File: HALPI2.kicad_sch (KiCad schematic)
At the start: 0 parts

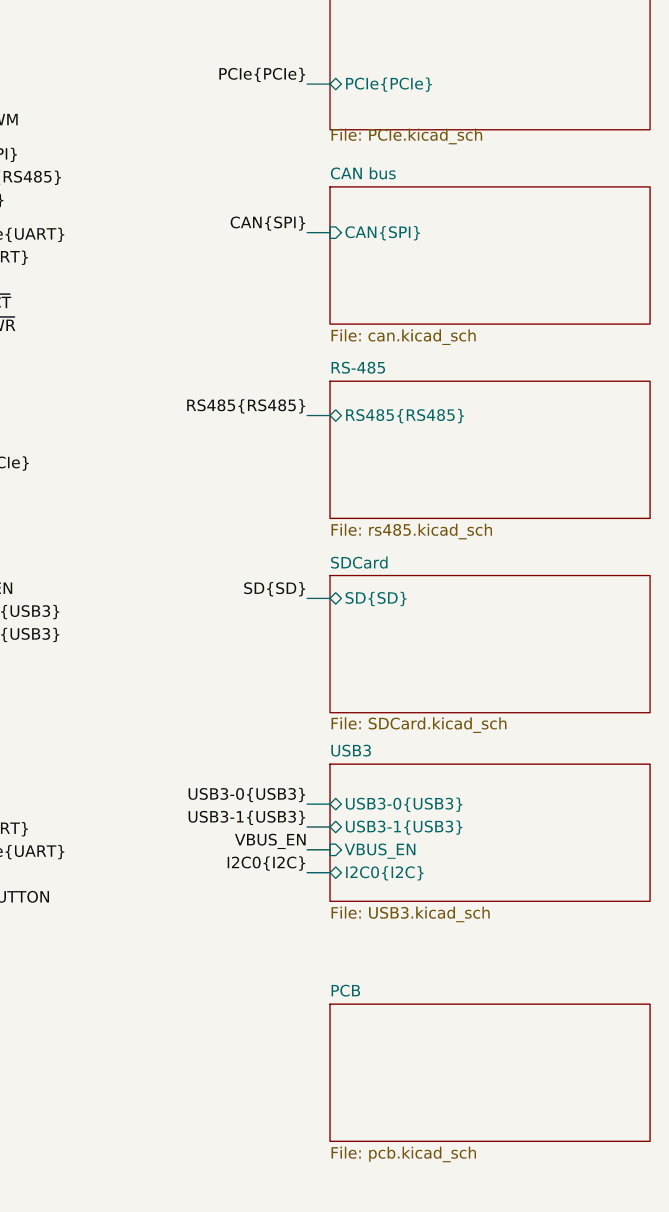
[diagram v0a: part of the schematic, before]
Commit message: Route more traces
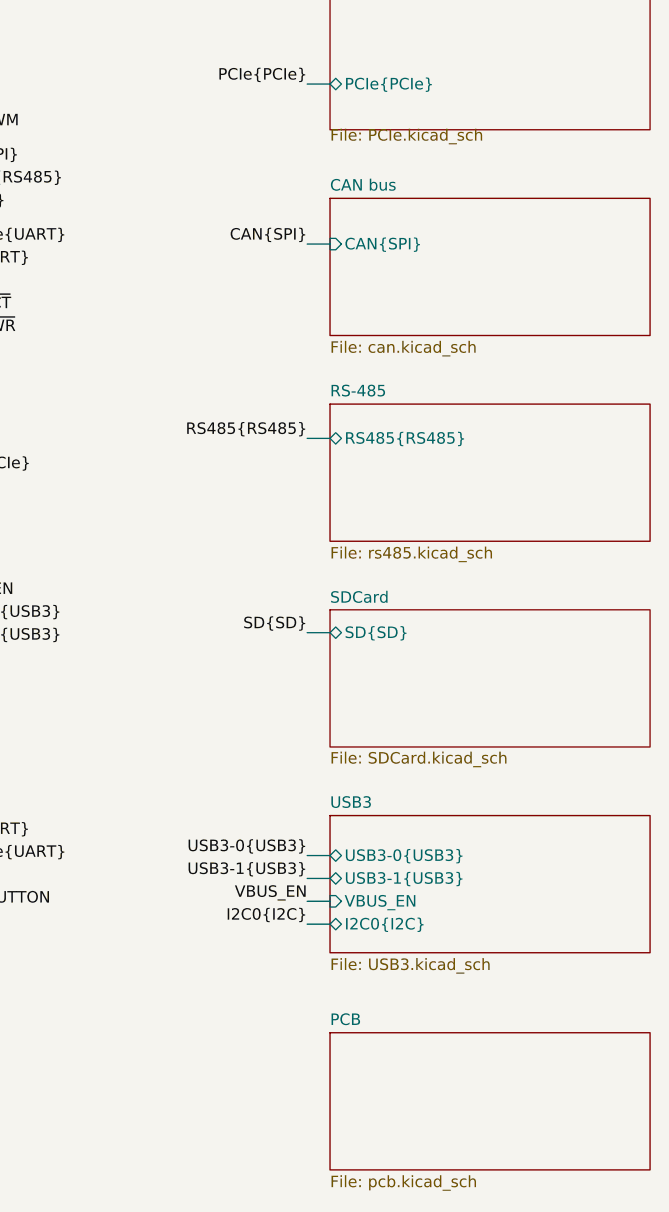
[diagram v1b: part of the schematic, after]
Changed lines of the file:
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@@
 	(bus
 		(pts
-			(xy 203.2 49.53) (xy 205.74 49.53)
-		)
-		(stroke
-			(width 0)
-			(type default)
-		)
-	)
-	(wire
-		(pts
-			(xy 203.2 118.11) (xy 205.74 118.11)
+			(xy 203.2 50.8) (xy 205.74 50.8)
+		)
+		(stroke
+			(width 0)
+			(type default)
+		)
+	)
+	(wire
+		(pts
+			(xy 203.2 123.825) (xy 205.74 123.825)
 		)
 		(stroke
@@
 	(bus
 		(pts
-			(xy 203.2 90.17) (xy 205.74 90.17)
+			(xy 203.2 93.98) (xy 205.74 93.98)
 		)
 		(stroke
@@
 	(bus
 		(pts
-			(xy 203.2 120.65) (xy 205.74 120.65)
+			(xy 203.2 126.365) (xy 205.74 126.365)
 		)
 		(stroke
@@
 	(bus
 		(pts
-			(xy 203.2 115.57) (xy 205.74 115.57)
+			(xy 203.2 121.285) (xy 205.74 121.285)
 		)
 		(stroke
@@
 	(bus
 		(pts
-			(xy 203.2 69.85) (xy 205.74 69.85)
+			(xy 203.2 72.39) (xy 205.74 72.39)
 		)
 		(stroke
@@
 	(bus
 		(pts
-			(xy 203.2 113.03) (xy 205.74 113.03)
+			(xy 203.2 118.745) (xy 205.74 118.745)
 		)
 		(stroke
@@
 	)
 	(label "SD{SD}"
-		(at 203.2 90.17 180)
+		(at 203.2 93.98 180)
 		(effects
 			(font
@@
 	)
 	(label "CAN{SPI}"
-		(at 203.2 49.53 180)
+		(at 203.2 50.8 180)
 		(effects
 			(font
@@
 	)
 	(label "RS485{RS485}"
-		(at 203.2 69.85 180)
+		(at 203.2 72.39 180)
 		(effects
 			(font
@@
 	)
 	(label "VBUS_EN"
-		(at 203.2 118.11 180)
+		(at 203.2 123.825 180)
 		(effects
 			(font
@@
 	)
 	(label "USB3-1{USB3}"
-		(at 203.2 115.57 180)
+		(at 203.2 121.285 180)
 		(effects
 			(font
@@
 	)
 	(label "USB3-0{USB3}"
-		(at 203.2 113.03 180)
+		(at 203.2 118.745 180)
 		(effects
 			(font
@@
 	)
 	(label "I2C0{I2C}"
-		(at 203.2 120.65 180)
+		(at 203.2 126.365 180)
 		(effects
 			(font
@@
 	)
 	(sheet
-		(at 205.74 66.04)
+		(at 205.74 68.58)
 		(size 35.56 15.24)
 		(exclude_from_sim no)
@@
 		)
 		(property "Sheetname" "RS-485"
-			(at 205.74 65.3284 0)
+			(at 205.74 67.8684 0)
 			(effects
 				(font
@@
 		)
 		(property "Sheetfile" "rs485.kicad_sch"
-			(at 205.74 81.8646 0)
+			(at 205.74 84.4046 0)
 			(effects
 				(font
@@
 		)
 		(pin "RS485{RS485}" bidirectional
-			(at 205.74 69.85 180)
+			(at 205.74 72.39 180)
 			(effects
 				(font
@@
 	)
 	(sheet
-		(at 205.74 44.45)
+		(at 205.74 45.72)
 		(size 35.56 15.24)
 		(exclude_from_sim no)
@@
 		)
 		(property "Sheetname" "CAN bus"
-			(at 205.74 43.7384 0)
+			(at 205.74 45.0084 0)
 			(effects
 				(font
@@
 		)
 		(property "Sheetfile" "can.kicad_sch"
-			(at 205.74 60.2746 0)
+			(at 205.74 61.5446 0)
 			(effects
 				(font
@@
 		)
 		(pin "CAN{SPI}" input
-			(at 205.74 49.53 180)
+			(at 205.74 50.8 180)
 			(effects
 				(font
@@
 	)
 	(sheet
-		(at 205.74 87.63)
+		(at 205.74 91.44)
 		(size 35.56 15.24)
 		(exclude_from_sim no)
@@
 		)
 		(property "Sheetname" "SDCard"
-			(at 205.74 86.9941 0)
+			(at 205.74 90.8041 0)
 			(effects
 				(font
@@
 		)
 		(property "Sheetfile" "SDCard.kicad_sch"
-			(at 205.74 103.3789 0)
+			(at 205.74 107.1889 0)
 			(effects
 				(font
@@
 		)
 		(pin "SD{SD}" bidirectional
-			(at 205.74 90.17 180)
+			(at 205.74 93.98 180)
 			(effects
 				(font
@@
 	)
 	(sheet
-		(at 205.74 108.585)
+		(at 205.74 114.3)
 		(size 35.56 15.24)
 		(exclude_from_sim no)
@@
 		)
 		(property "Sheetname" "USB3"
-			(at 205.74 107.8734 0)
+			(at 205.74 113.5884 0)
 			(effects
 				(font
@@
 		)
 		(property "Sheetfile" "USB3.kicad_sch"
-			(at 205.74 124.4096 0)
+			(at 205.74 130.1246 0)
 			(effects
 				(font
@@
 		)
 		(pin "USB3-0{USB3}" bidirectional
-			(at 205.74 113.03 180)
+			(at 205.74 118.745 180)
 			(effects
 				(font
@@
 		)
 		(pin "USB3-1{USB3}" bidirectional
-			(at 205.74 115.57 180)
+			(at 205.74 121.285 180)
 			(effects
 				(font
@@
 		)
 		(pin "VBUS_EN" input
-			(at 205.74 118.11 180)
+			(at 205.74 123.825 180)
 			(effects
 				(font
@@
 		)
 		(pin "I2C0{I2C}" bidirectional
-			(at 205.74 120.65 180)
+			(at 205.74 126.365 180)
 			(effects
 				(font
@@
 	)
 	(sheet
-		(at 205.74 135.255)
+		(at 205.74 138.43)
 		(size 35.56 15.24)
 		(exclude_from_sim no)
@@
 		)
 		(property "Sheetname" "PCB"
-			(at 205.74 134.5434 0)
+			(at 205.74 137.7184 0)
 			(effects
 				(font
@@
 		)
 		(property "Sheetfile" "pcb.kicad_sch"
-			(at 205.74 151.0796 0)
-			(effects
-				(font
+			(at 205.74 154.2546 0)
+			(effects
+				(font
